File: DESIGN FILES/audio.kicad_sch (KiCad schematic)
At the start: 22 parts, among them J701 PJ-342B-TX-SMT, J702 PJ-342B-TX-SMT, J703 PJ-342B-TX-SMT, U701 WM8978CGEFL_RV

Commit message: up
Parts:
- R704, R705: footprint MY RESISTOR LIBRARY:0805W8F1000T5E -> MY RESISTOR LIBRARY:0603WAF1000T5E
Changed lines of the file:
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@@
     (property "Reference" "R704" (id 0) (at 278.13 154.94 90))
     (property "Value" "100R" (id 1) (at 278.13 160.02 90))
-    (property "Footprint" "MY RESISTOR LIBRARY:0805W8F1000T5E" (id 2) (at 278.13 159.258 90)
+    (property "Footprint" "MY RESISTOR LIBRARY:0603WAF1000T5E" (id 2) (at 278.13 159.258 90)
       (effects (font (size 1.27 1.27)) hide)
     )
@@
     (property "Reference" "R705" (id 0) (at 278.13 162.56 90))
     (property "Value" "100R" (id 1) (at 278.13 167.64 90))
-    (property "Footprint" "MY RESISTOR LIBRARY:0805W8F1000T5E" (id 2) (at 278.13 166.878 90)
-      (effects (font (size 1.27 1.27)) hide)
-    )
+    (property "Footprint" "MY RESISTOR LIBRARY:0603WAF1000T5E" (id 2) (at 278.13 166.878 90)
+      (effects (font (size 1.27 1.27)) hide)
+    )

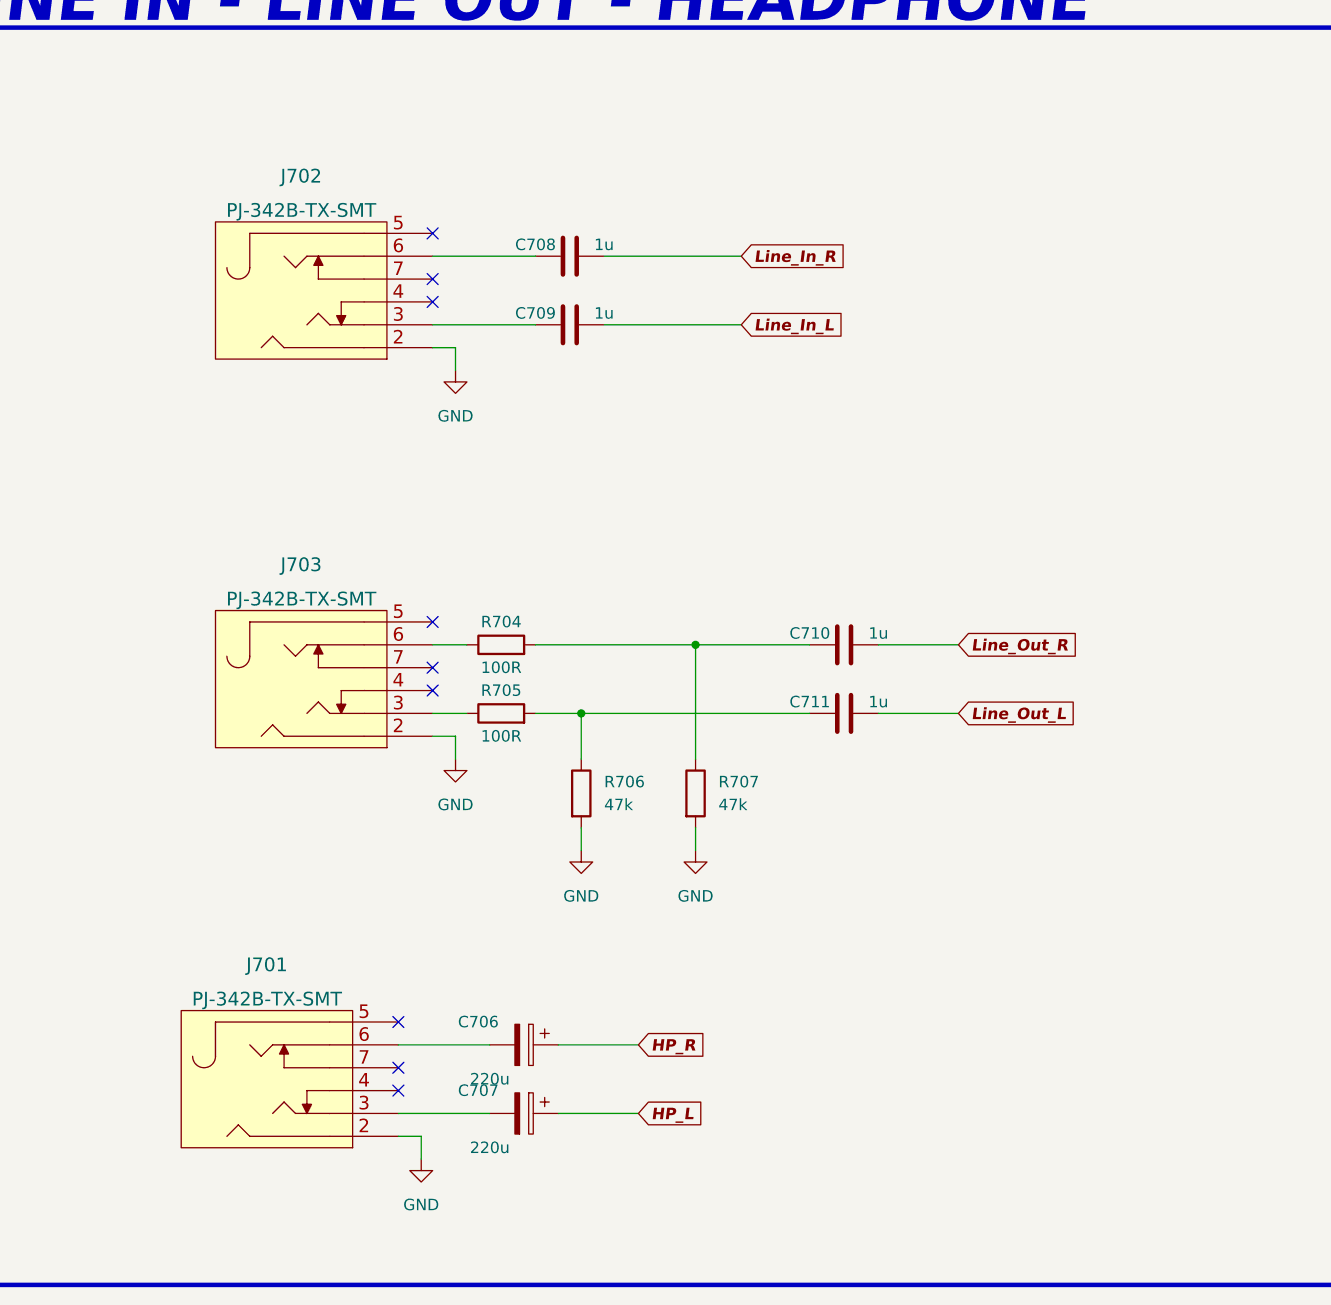
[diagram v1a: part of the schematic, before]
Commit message: updates
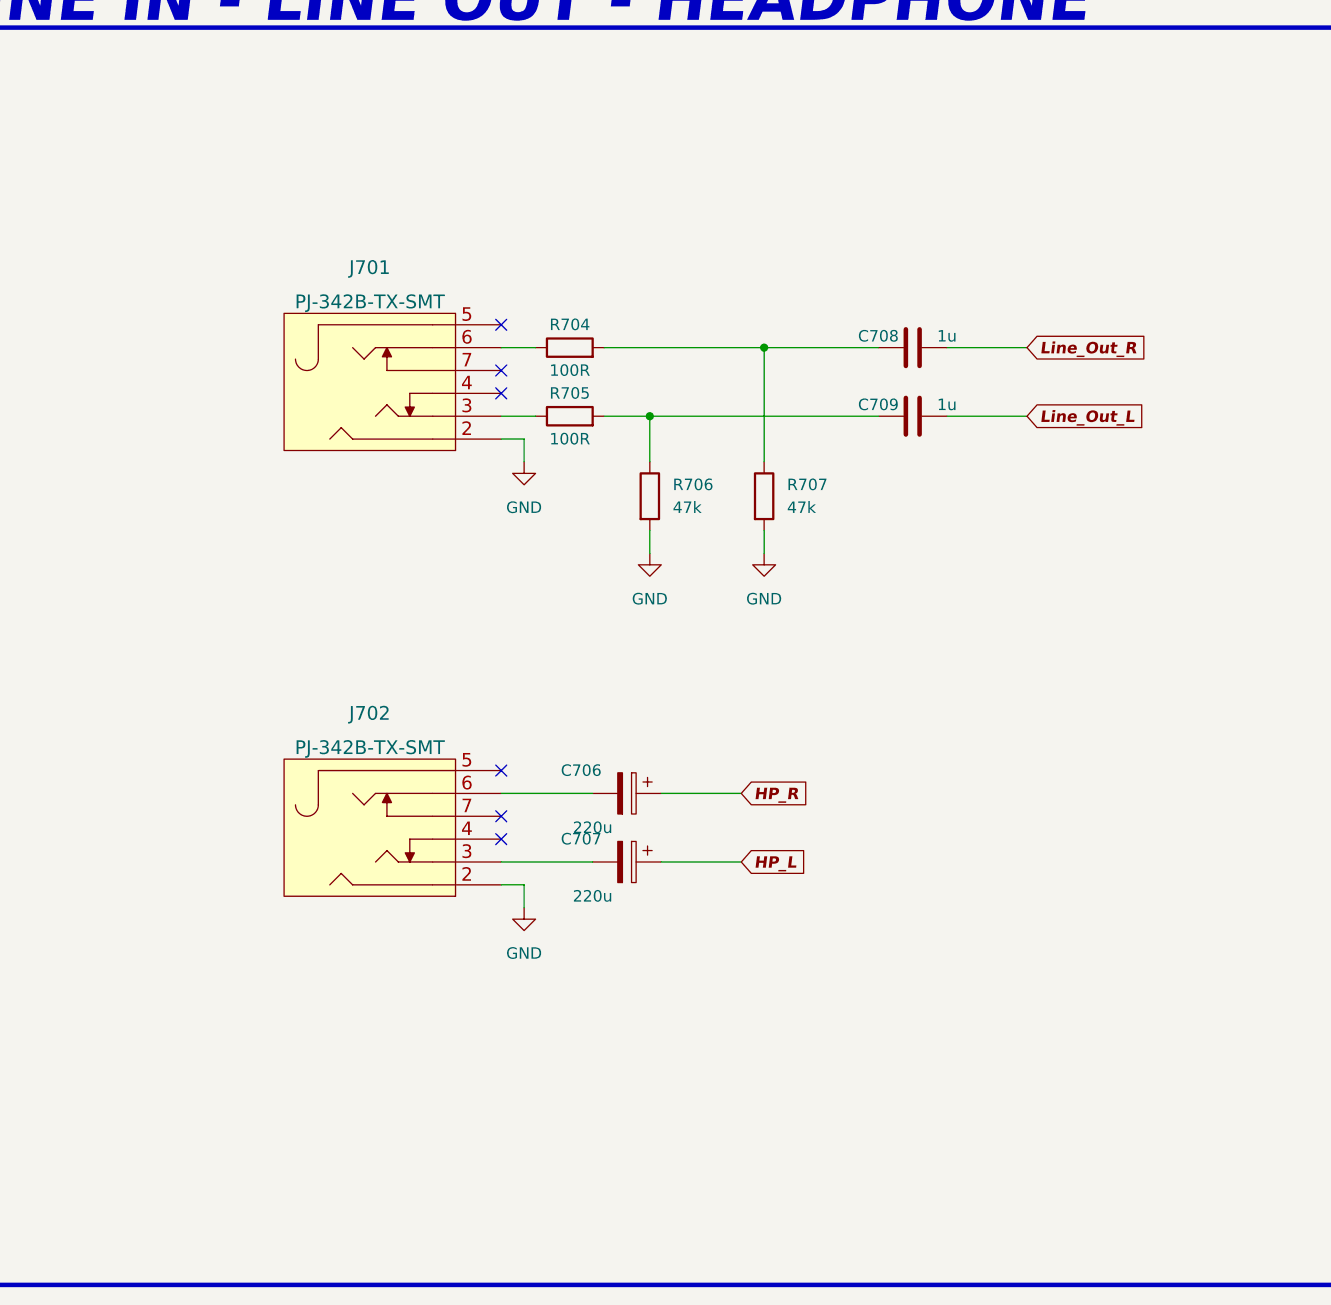
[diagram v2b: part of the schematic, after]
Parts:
- removed C708, C709: 1u, MY CAPACITOR LIBRARY:0402_CL05A105KA5NQNC, symbol MY CAPACITOR LIBRARY:CL05A105KA5NQNC
- removed J702: PJ-342B-TX-SMT, MY CONNECTOR LIBRARY:PJ-342B-TX-SMT, symbol MY CONNECTOR LIBRARY:PJ-342B-TX-SMT
- renumbered C710 to C708, C711 to C709, J703 to J701, J701 to J702
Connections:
- no-connect marks 19 -> 16
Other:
- moved on the sheet: C706, C707, C708, C709, J701, J702, R704, R705, R706, R707
